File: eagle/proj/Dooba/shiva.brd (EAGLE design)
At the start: 83.7 x 53.3 mm, 114 parts, among them J1 DM3D-SFDM, J2 USB-BAMPHENOL-MICRO, J3 SJ1-3523N, J4 ADAFRUIT_OLED_13, P1 PB[2-3-4], P2 PB5-PB6/SCL-PB7/SDA, P3 PB[8-9-10], P4 PF6-PF7-PA8, P5 PA[11-12-15], P6 PA13/SWDIO-PA14/SWCLK-RST, P7 5.5V-USBVCC-GND, P8 5.5V-BATTVCC-GND, P9 AOUT_L-GND-AOUT_R, SW1 VD, SW2 D, SW3 R, SW4 VU, SW5 C, SW6 U, SW7 L, U1 STM32F030X-LQFP48LQFP48, U10 CS4334, U11 LM4811PDSO-10, U12 5.0V, U13 MCP23008QFN, U2 TPS61200S-PVSON-N10, U3 MAX1811SO8, U4 FT232RQFN32, U5 SN74LVC1G125SOT23-5, U6 SN74LVC1G125SOT23-5, U7 3.3V, U8 3.3V, U9 STA013LQFP44, X1 16MHz, X2 14.7456MHz

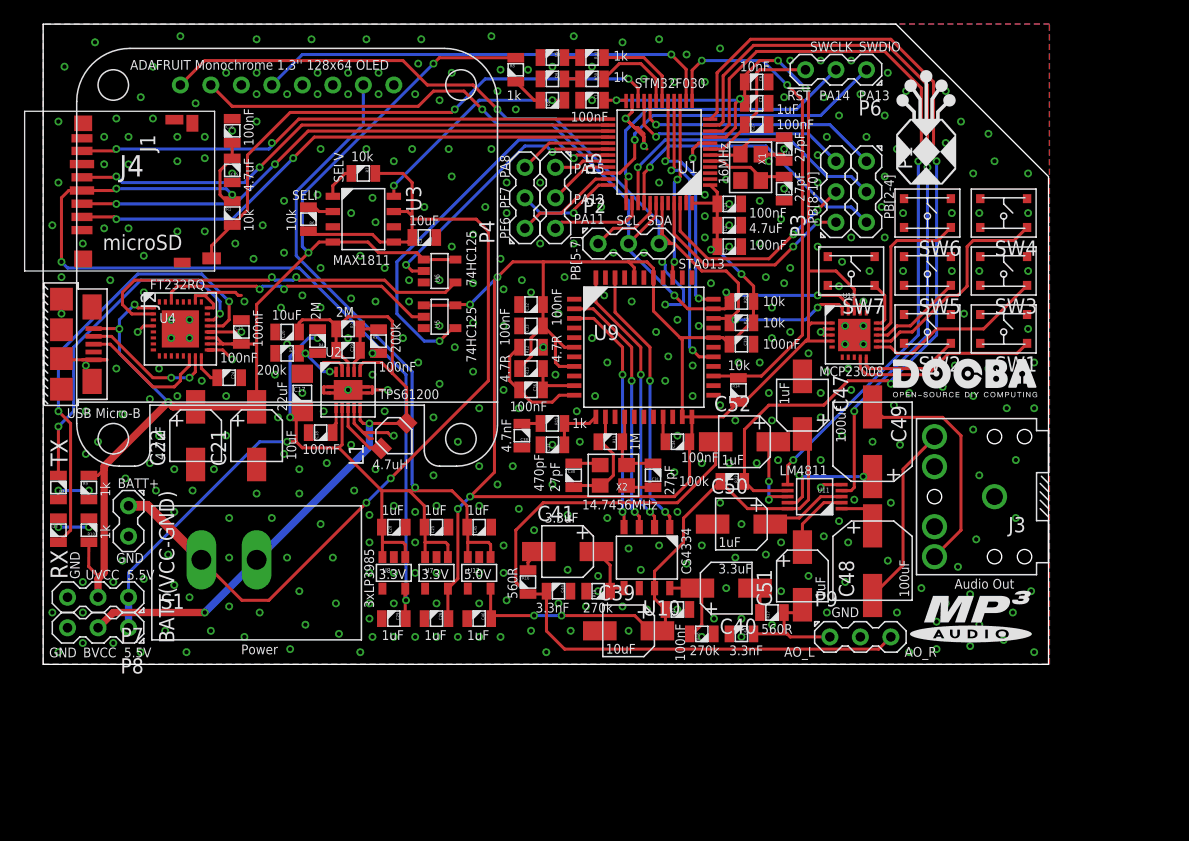
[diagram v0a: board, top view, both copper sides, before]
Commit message: Started designing Shiva mp3 player (new version)
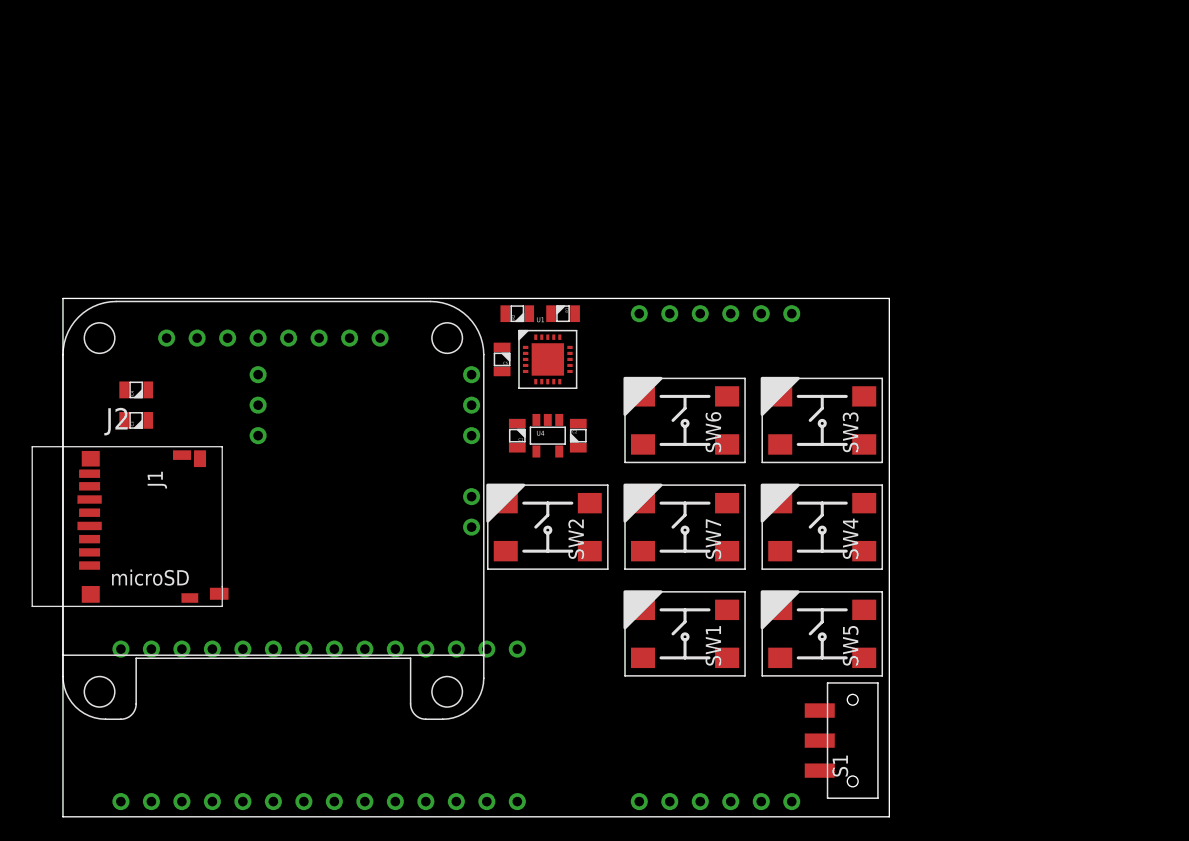
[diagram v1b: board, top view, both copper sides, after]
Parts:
- removed BATT(VCC-GND): PIN_2, dooba:PIN_2
- removed C10, C30, C31, C9: 27pF, dooba:0805
- removed C11, C16, C18, C19, C23, C24, C27, C32, C33, C34, C35, C36, C42: 100nF, dooba:0805
- removed C15, C8: 4.7uF, dooba:0805
- removed C17: 22uF, dooba:1206
- removed C20: 10uF, dooba:0805
- removed C21, C39: 10uF, dooba:RADCAP_SMD_43
- removed C22: 4.7uF, dooba:RADCAP_SMD_43
- removed C25, C26, C28, C29, C45, C46, C7: 1uF, dooba:0805
- removed C37: 470pF, dooba:0805
- removed C38: 4.7nF, dooba:0805
- removed C40, C41: 3.3uF, dooba:RADCAP_SMD_43
- removed C43, C44: 3.3nF, dooba:0805
- removed C47, C50, C51, C52: 1uF, dooba:RADCAP_SMD_43
- removed C48, C49: 100uF, dooba:RADCAP_SMD_66
- removed C6: 10nF, dooba:0805
- removed D1: CHARGE, dooba:0805
- removed D2: TX, dooba:0805
- removed D3: RX, dooba:0805
- removed D4: MicroSD, dooba:0805
- removed D5: Activity, dooba:0805
- removed J3: SJ1-3523N, dooba:SJ1-352XN
- removed J4: ADAFRUIT_OLED_13, dooba:ADAFRUIT_OLED_13
- removed L1: 4.7uH, dooba:IND-SMD-3232
- removed P1: PB[2-3-4], dooba:PIN_3
- removed P2: PB5-PB6/SCL-PB7/SDA, dooba:PIN_3
- removed P3: PB[8-9-10], dooba:PIN_3
- removed P4: PF6-PF7-PA8, dooba:PIN_3
- removed P5: PA[11-12-15], dooba:PIN_3
- removed P6: PA13/SWDIO-PA14/SWCLK-RST, dooba:PIN_3
- removed P7: 5.5V-USBVCC-GND, dooba:PIN_3
- removed P8: 5.5V-BATTVCC-GND, dooba:PIN_3
- removed P9: AOUT_L-GND-AOUT_R, dooba:PIN_3
- removed R10, R15, R30, R31, R8, R9: 1k, dooba:0805
- removed R11: 1M, dooba:0805
- removed R12, R13: 4.7R, dooba:0805
- removed R14, R20, R21, R6, R7: 10k, dooba:0805
- removed R16, R17: 560R, dooba:0805
- removed R18, R19: 270k, dooba:0805
- removed R22: 100k, dooba:0805
- removed R3, R5: 200k, dooba:0805
- removed R4: 2M, dooba:0805
- removed U10: CS4334, dooba:SO8
- removed U11: LM4811PDSO-10, dooba:PDSO-10
- removed U12: 5.0V, dooba:SOT23-5
- removed U13: MCP23008QFN, dooba:20-VQFN
- removed U5, U6: SN74LVC1G125SOT23-5, dooba:SOT23-5
- removed U7, U8: 3.3V, dooba:SOT23-5
- removed U9: STA013LQFP44, dooba:QFP44
- removed X1: 16MHz, dooba:XTAL_3225
- removed X2: 14.7456MHz, dooba:XTAL_3225
- added C3: 10uF, dooba:0805
- added C4: 100nF, dooba:0805
- added N1: DOOBA_IONODE, dooba:DOOBA_IONODE
- C1: value 100nF -> 1uF
- C2: value 10uF -> 1uF
- J2: value USB-BAMPHENOL-MICRO -> ADAFRUIT_OLED_13; device dooba:AMPHENOL-USB-MICRO-B -> dooba:ADAFRUIT_OLED_13
- R2: value 2M -> 10k
- S1: value SWITCH_SPSTGF-1123-0025 -> PWR; device dooba:GF-1123-0025 -> dooba:JS102011
- SW1: value VD -> TACTSWB3SL-10XXP; device dooba:TACTSW_CK_PTS_830 -> dooba:B3SL-10XXP
- SW2: value D -> TACTSWB3SL-10XXP; device dooba:TACTSW_CK_PTS_830 -> dooba:B3SL-10XXP
- SW3: value R -> TACTSWB3SL-10XXP; device dooba:TACTSW_CK_PTS_830 -> dooba:B3SL-10XXP
- SW4: value VU -> TACTSWB3SL-10XXP; device dooba:TACTSW_CK_PTS_830 -> dooba:B3SL-10XXP
- SW5: value C -> TACTSWB3SL-10XXP; device dooba:TACTSW_CK_PTS_830 -> dooba:B3SL-10XXP
- SW6: value U -> TACTSWB3SL-10XXP; device dooba:TACTSW_CK_PTS_830 -> dooba:B3SL-10XXP
- SW7: value L -> TACTSWB3SL-10XXP; device dooba:TACTSW_CK_PTS_830 -> dooba:B3SL-10XXP
- U1: value STM32F030X-LQFP48LQFP48 -> MCP23008QFN; device dooba:QFP48 -> dooba:20-VQFN
- U2: value TPS61200S-PVSON-N10 -> DOOBA_AECHO_NOAOUT; device dooba:S-PVSON-N10 -> dooba:DOOBA_AECHO_NOAOUT
- U3: value MAX1811SO8 -> DOOBA_NOMAD; device dooba:SO8 -> dooba:DOOBA_NOMAD
- U4: value FT232RQFN32 -> 3.3V; device dooba:32-VQFN -> dooba:SOT23-5
- moved S1 51.6 mm to (73.7, 24.1), turned to 90 degrees
- moved SW1 36.7 mm to (59.7, 33.0), turned to 0 degrees
- moved SW2 35.7 mm to (48.3, 41.9), turned to 0 degrees
- moved U2 33.6 mm to (62.2, 39.4), flipped to the bottom, turned to 270 degrees
- moved U4 31.9 mm to (48.3, 49.5)
- moved SW5 31.5 mm to (71.1, 33.0), turned to 0 degrees
- moved SW4 30.2 mm to (71.1, 41.9), turned to 0 degrees
- moved R1 28.8 mm to (49.5, 59.7), turned to 180 degrees
- moved C1 28.6 mm to (45.7, 49.5), turned to 90 degrees
- moved J1 27.9 mm to (11.4, 41.9)
- moved SW6 26.6 mm to (59.7, 50.8), turned to 0 degrees
- moved SW7 25.4 mm to (59.7, 41.9), turned to 0 degrees
- moved C5 21.1 mm to (44.5, 55.9), turned to 90 degrees
- moved C2 20.9 mm to (50.8, 49.5), turned to 270 degrees
- moved U1 19.6 mm to (48.3, 55.9), turned to 0 degrees
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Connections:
- removed net !MICROSD_CS: J1.DAT3/CS, U1.28
- removed net !STA013_RST: R14.1, U1.13, U9.25
- removed net 3.3V-CORE: C1.1, C11.1, C26.1, C32.2, C33.2, C34.2, C35.2, C5.1, C6.2, C7.2, C8.1, R13.1, R14.2, R20.1, R21.1, U1.1, U1.24, U1.48, U1.9, U13.1, U13.18, U13.4, U5.1, U5.5, U7.5, U9.21, U9.22, U9.29, U9.38, U9.40, U9.6, U9.8
- removed net 3.3V-MICROSD: C15.2, C16.2, C29.1, J1.VDD, R1.1, U8.5
- removed net 5.0V-AUDIO: C39.2, C42.1, C46.1, C47.2, R22.2, U10.P$7, U11.10, U12.5
- removed net AMP_SHUTDOWN: R22.1, U1.12, U11.7
- removed net AMP_VOL_CLK: U1.11, U11.4
- removed net AMP_VOL_UPDN: U1.10, U11.6
- removed net AOUT_L: C43.1, C51.1, P9.1, R17.2
- removed net AOUT_R: C44.2, C52.1, P9.3, R16.2
- removed net BATTVCC: C19.2, C20.2, L1.2, P8.2, R2.2, S1.2, U2.5, U2.6, U2.8
- removed net BATT_PWR: BATT(VCC-GND).1, C2.1, R6.1, R7.1, S1.1, U3.P$5, U3.P$7
- removed net FT232R_RX: U4.P$2, U6.4
- removed net FT232R_TX: U4.P$30, U5.2
- removed net MICROSD_DET: J1.SW_A, R1.2, U1.22
- removed net N$10: C40.2, R18.1, U10.P$8
- removed net N$12: C41.2, R19.2, U10.P$5
- removed net N$13: C19.1, R2.1, R3.1, U2.7
- removed net N$14: R4.1, R5.1, U2.10
- removed net N$15: C18.2, U2.1
- removed net N$16: L1.1, U2.3
- removed net N$17: D1.2, U3.P$8
- removed net N$18: D1.1, R8.2
- removed net N$19: R7.2, U3.P$1
- removed net N$20: R6.2, U3.P$2
- removed net N$21: C24.2, U4.P$16
- removed net N$22: D2.2, U4.P$22
- removed net N$23: D3.2, U4.P$21
- removed net N$24: D2.1, R9.2
- removed net N$25: D3.1, R10.2
- removed net N$26: J2.2, U4.P$15
- removed net N$27: J2.3, U4.P$14
- removed net N$28: C41.1, R16.1
- removed net N$29: C40.1, R17.1
- removed net N$30: C48.2, U11.1
- removed net N$31: C49.2, U11.9
- removed net N$32: C50.2, U11.3
- removed net N$33: SW1.1, U13.9
- removed net N$34: C49.1, J3.3
- removed net N$35: SW2.1, U13.10
- removed net N$36: SW3.1, U13.11
- removed net N$37: SW4.1, U13.12
- removed net N$38: SW5.1, U13.13
- removed net N$39: C51.2, U11.2
- removed net N$40: C52.2, U11.8
- removed net N$41: SW6.1, U13.14
- removed net N$42: SW7.1, U13.15
- removed net N$43: D4.1, R30.2
- removed net N$44: D5.1, R31.2
- removed net N$45: R30.1, U1.19
- removed net N$46: R31.1, U1.18
- removed net N$47: P3.3, U1.21
- removed net N$48: P3.2, U1.46
- removed net N$49: P3.1, U1.45
- removed net N$50: P2.1, U1.41
- removed net N$51: P1.3, U1.40
- removed net N$52: P1.2, U1.39
- removed net N$53: P1.1, U1.20
- removed net N$54: P4.3, U1.29
- removed net N$55: P4.1, U1.35
- removed net N$56: P4.2, U1.36
- removed net N$57: P5.1, U1.32
- removed net N$58: P5.2, U1.33
- removed net N$59: P5.3, U1.38
- removed net N$60: P6.1, U1.34
- removed net N$61: P6.2, U1.37
- removed net N$8: C48.1, J3.2
- removed net N$9: C38.2, R15.2
- removed net STA013_DREQ: U1.16, U9.27
- removed net STA013_LRCKT: U10.P$3, U9.2
- removed net STA013_OCLK: U10.P$4, U9.3
- removed net STA013_SCKR: U1.15, U9.36
- removed net STA013_SCKT: U10.P$2, U9.44
- removed net STA013_SDI: U1.17, U9.33
- removed net STA013_SDO: U10.P$1, U9.42
- removed net STM32F0_RX: U1.31, U5.4
- removed net STM32F0_TX: U1.30, U6.2
- removed net USBVCC: C21.2, C22.2, C23.2, J2.1, P7.2, R10.1, R8.1, R9.1, U3.P$4, U4.P$1, U4.P$18, U4.P$19, U6.1, U6.5
- new net 3.3V: C2.2, C3.1, C4.1, C5.1, J1.VDD, R1.2, R2.2, U1.1, U1.18, U1.4, U4.5
- new net AMP_CLK: N1.19, U2.5
- new net AMP_SHDN: N1.20, U2.4
- new net AMP_VUPDN: N1.18, U2.6
- new net MICROSD_CS: J1.DAT3/CS, N1.14
- new net MP3_DREQ: N1.27, U2.8
- new net MP3_RST: N1.28, U2.7
- new net MP3_SCKR: N1.25, U2.10
- new net MP3_SDI: N1.26, U2.9
- new net VBAT: S1.2, U3.10
- new net VUSB: N1.2, U3.4
- net 5.5V: now also C1.2, J2.VIN, N1.15, U3.3, U3.8, U4.1, U4.3; no longer C17.2, C25.1, C28.1, C45.1, J4.VIN, P7.1, P8.1, R4.2, U12.1, U12.3, U7.1, U7.3, U8.1, U8.3
- net GND: now also C1.1, C2.1, C3.2, C4.2, J2.GND, N1.1, N1.16, U1.17, U1.2, U1.3, U1.PAD, U2.1, U2.3, U3.5, U3.6, U3.9, U4.2; no longer BATT(VCC-GND).2, C1.2, C10.1, C11.2, C15.1, C16.1, C17.1, C18.1, C2.2, C20.1, C21.1, C22.1, C23.1, C24.1, C25.2, C26.2, C27.2, C28.2, C29.2, C30.1, C31.1, C32.1, C33.1, C34.1, C35.1, C37.1, C38.1, C39.1, C42.2, C43.2, C44.1, C45.2, C46.2, C47.1, C50.1, C6.1, C7.1, C8.2, C9.1, D4.2, D5.2, J1.SW_B, J2.5, J2.P$10, J2.P$11, J2.P$6, J2.P$7, J2.P$8, J2.P$9, J3.1, J4.GND, P7.3, P8.3, P9.2, R12.2, R18.2, R19.1, R3.2, R5.2, U1.23, U1.47, U1.8, U10.P$6, U11.5, U12.2, U13.17, U13.2, U13.3, U13.PAD, U2.4, U2.9, U2.PAD, U2.PAD0, U2.PAD1, U2.PAD2, U2.PAD3, U3.P$3, U3.P$6, U4.P$17, U4.P$20, U4.P$24, U4.P$26, U4.P$33, U4.P$4, U5.3, U6.3, U7.2, U8.2, U9.19, U9.24, U9.26, U9.30, U9.5, U9.7, X1.2, X1.4, X2.2, X2.4
- net I2C_SCL: now also J2.CLK, N1.21, R1.1, U1.19, U2.12; no longer J4.CLK, P2.2, R20.2, U1.42, U13.19, U9.32
- net I2C_SDA: now also J2.DATA, N1.22, R2.1, U1.20, U2.11; no longer J4.DATA, P2.3, R21.2, U1.43, U13.20, U9.31
- net MICROSD_MISO: now also N1.11; no longer U1.25
- net MICROSD_MOSI: now also N1.13; no longer U1.27
- net MICROSD_SCK: now also N1.12; no longer U1.26
- net N$1: now also SW1.1, U1.9; no longer C27.1, P6.3, U1.7
- net N$11: now also S1.1, U3.7; no longer C37.2, R15.1, U9.12
- net N$2: now also SW2.1, U1.10; no longer C31.2, R11.1, U9.15, X2.1
- net N$3: now also SW3.1, U1.11; no longer C30.2, R11.2, U9.13, X2.3
- net N$4: now also SW4.1, U1.12; no longer C9.2, U1.5, X1.3
- net N$5: now also SW5.1, U1.13; no longer C10.2, U1.6, X1.1
- net N$6: now also SW6.1, U1.14; no longer C36.1, R13.2, U9.10
- net N$7: now also SW7.1, U1.15; no longer C36.2, R12.1, U9.11
- net OLED_RST: now also J2.RST, N1.17; no longer J4.RST, U1.14
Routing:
- net 3.3V-CORE: track 201.7 -> 0.00 mm, vias 10 -> 0
- net 5.5V: track 120.1 -> 0.00 mm, vias 4 -> 0
- net USBVCC: track 106.4 -> 0.00 mm, vias 5 -> 0
- net 3.3V-MICROSD: track 81.6 -> 0.00 mm, vias 4 -> 0
- net BATT_PWR: track 78.9 -> 0.00 mm, vias 2 -> 0
- net I2C_SDA: track 76.4 -> 0.00 mm, vias 3 -> 0
- net AMP_SHUTDOWN: track 73.8 -> 0.00 mm, vias 2 -> 0
- net I2C_SCL: track 71.5 -> 0.00 mm, vias 4 -> 0
- net GND: track 71.3 -> 0.00 mm, vias 420 -> 0
- net BATTVCC: track 62.2 -> 0.00 mm, vias 2 -> 0
- net AMP_VOL_CLK: track 61.7 -> 0.00 mm, vias 2 -> 0
- net AMP_VOL_UPDN: track 61.5 -> 0.00 mm, vias 2 -> 0
- net AOUT_R: track 61.2 -> 0.00 mm
- net !MICROSD_CS: track 46.7 -> 0.00 mm, vias 2 -> 0
- net 5.0V-AUDIO: track 46.6 -> 0.00 mm, vias 2 -> 0
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- removed copper zone on layer 1, net GND
- removed copper zone on layer 16, net GND
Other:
- board size 83.7 x 53.3 mm -> 68.8 x 43.2 mm
- board text removed: "!RST"
- board text removed: "100k"
- board text removed: "100nF"
- board text removed: "100uF"
- board text removed: "10k"
- board text removed: "10nF"
- board text removed: "10uF"
- board text removed: "14.7456MHz"
- board text removed: "16MHz"
- board text removed: "1M"
- board text removed: "1k"
- board text removed: "1uF"
- board text removed: "200k"
- board text removed: "22uF"
- board text removed: "270k"
- board text removed: "27pF"
- board text removed: "2M"
- board text removed: "3.3V"
- board text removed: "3.3nF"
- board text removed: "3.3uF"
- board text removed: "3xLP3985"
- board text removed: "4.7R"
- board text removed: "4.7nF"
- board text removed: "4.7uF"
- board text removed: "4.7uH"
- board text removed: "470pF"
- board text removed: "5.0V"
- board text removed: "5.5V"
- board text removed: "560R"
- board text removed: "74HC125"
- board text removed: "ADAFRUIT Monochrome 1.3'' 128x64 OLED"
- board text removed: "AO_L"
- board text removed: "AO_R"
- board text removed: "Audio Out"
- board text removed: "BATT+"
- board text removed: "BVCC"
- board text removed: "CS4334"
- board text removed: "FT232RQ"
- board text removed: "GND"
- board text removed: "LM4811"
- board text removed: "MAX1811"
- board text removed: "MCP23008"
- board text removed: "PA11"
- board text removed: "PA12"
- board text removed: "PA13"
- board text removed: "PA14"
- board text removed: "PA15"
- board text removed: "PA8"
- board text removed: "PB[2-4]"
- board text removed: "PB[5-7]"
- board text removed: "PB[8-10]"
- board text removed: "PF6"
- board text removed: "PF7"
- board text removed: "Power"
- board text removed: "RX"
- board text removed: "SCL"
- board text removed: "SDA"
- board text removed: "SELI"
- board text removed: "SELV"
- board text removed: "STA013"
- board text removed: "STM32F030"
- board text removed: "SWCLK"
- board text removed: "SWDIO"
- board text removed: "TPS61200"
- board text removed: "TX"
- board text removed: "USB Micro-B"
- board text removed: "UVCC"

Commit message: Finished Shiva board
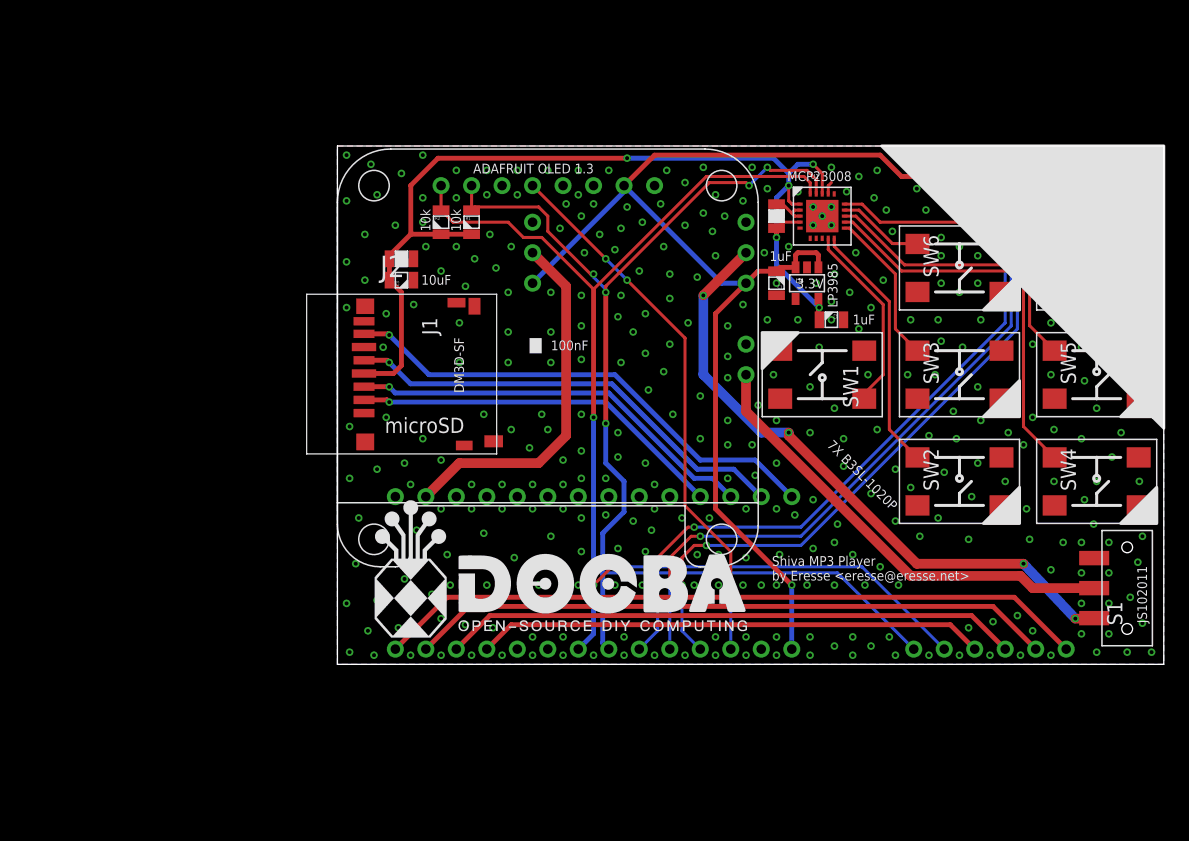
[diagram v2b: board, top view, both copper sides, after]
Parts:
- moved SW7 40.5 mm to (94.0, 63.5), turned to 180 degrees
- moved SW2 34.5 mm to (82.5, 45.7), turned to 180 degrees
- moved SW5 31.4 mm to (94.0, 54.6), turned to 180 degrees
- moved U2 26.2 mm to (85.1, 52.1)
- moved J1 26.2 mm to (34.3, 54.6)
- moved J2 26.2 mm to (48.3, 70.4)
- moved N1 26.2 mm to (52.1, 38.1)
- moved S1 26.2 mm to (96.5, 36.8)
- moved SW6 26.2 mm to (82.5, 63.5), turned to 180 degrees
- moved U3 26.2 mm to (55.9, 61.0)
- moved U1 25.8 mm to (71.1, 67.8)
- moved C5 25.8 mm to (67.3, 67.8)
- moved C1 25.0 mm to (67.3, 62.2)
- moved U4 25.0 mm to (69.8, 62.2)
- moved C3 25.0 mm to (36.1, 62.5)
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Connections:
- net MICROSD_CS: now also N1.11; no longer N1.14
- net MICROSD_MISO: now also N1.14; no longer N1.11
- net MICROSD_MOSI: now also N1.12; no longer N1.13
- net MICROSD_SCK: now also N1.13; no longer N1.12
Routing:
- net I2C_SDA: track 0.00 -> 104.0 mm, vias 0 -> 3
- net I2C_SCL: track 0.00 -> 101.1 mm, vias 0 -> 5
- net 5.5V: track 0.00 -> 96.8 mm, vias 0 -> 1
- net 3.3V: track 0.00 -> 83.6 mm, vias 0 -> 5
- net AMP_VUPDN: track 0.00 -> 59.7 mm, vias 0 -> 2
- net MP3_RST: track 0.00 -> 59.5 mm
- net AMP_SHDN: track 0.00 -> 58.8 mm, vias 0 -> 2
- net AMP_CLK: track 0.00 -> 58.6 mm, vias 0 -> 2
- net MP3_DREQ: track 0.00 -> 53.7 mm
- net N$11: track 0.00 -> 52.8 mm, vias 0 -> 4
- net MP3_SDI: track 0.00 -> 48.0 mm
- net OLED_RST: track 0.00 -> 45.4 mm, vias 0 -> 3
- net MP3_SCKR: track 0.00 -> 42.3 mm
- net MICROSD_MISO: track 0.00 -> 41.2 mm, vias 0 -> 1
- net VBAT: track 0.00 -> 38.2 mm
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- added copper zone on layer 1, net GND
- added copper zone on layer 16, net GND
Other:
- board text added: "100nF"
- board text added: "10k"
- board text added: "10uF"
- board text added: "1uF"
- board text added: "3.3V"
- board text added: "7X B3SL-1020P"
- board text added: "ADAFRUIT OLED 1.3"
- board text added: "Aecho"
- board text added: "DM3D-SF"
- board text added: "JS102011"
- board text added: "LP3985"
- board text added: "MCP23008"
- board text added: "Nomad"
- board text added: "Shiva MP3 Player by Eresse <eresse@eresse.net>"
- board text added: "ioNode"
